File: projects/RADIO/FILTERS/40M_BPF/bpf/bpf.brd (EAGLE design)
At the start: 90 x 30 mm, 15 parts

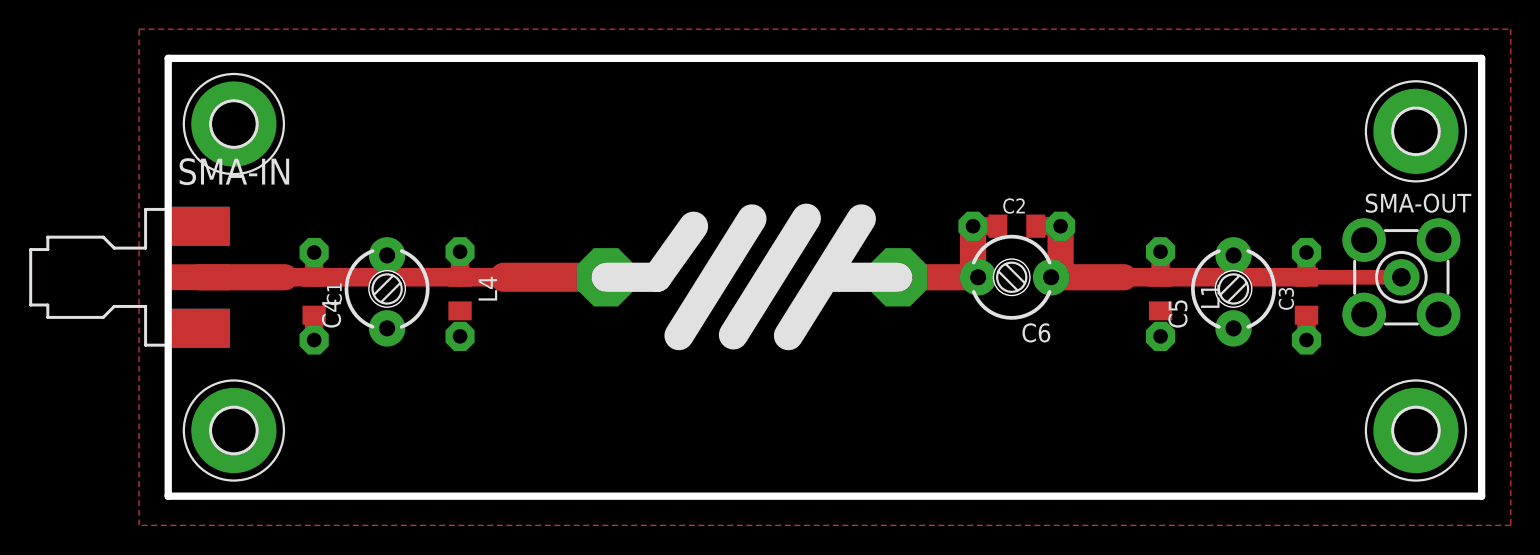
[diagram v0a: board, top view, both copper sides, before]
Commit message: update
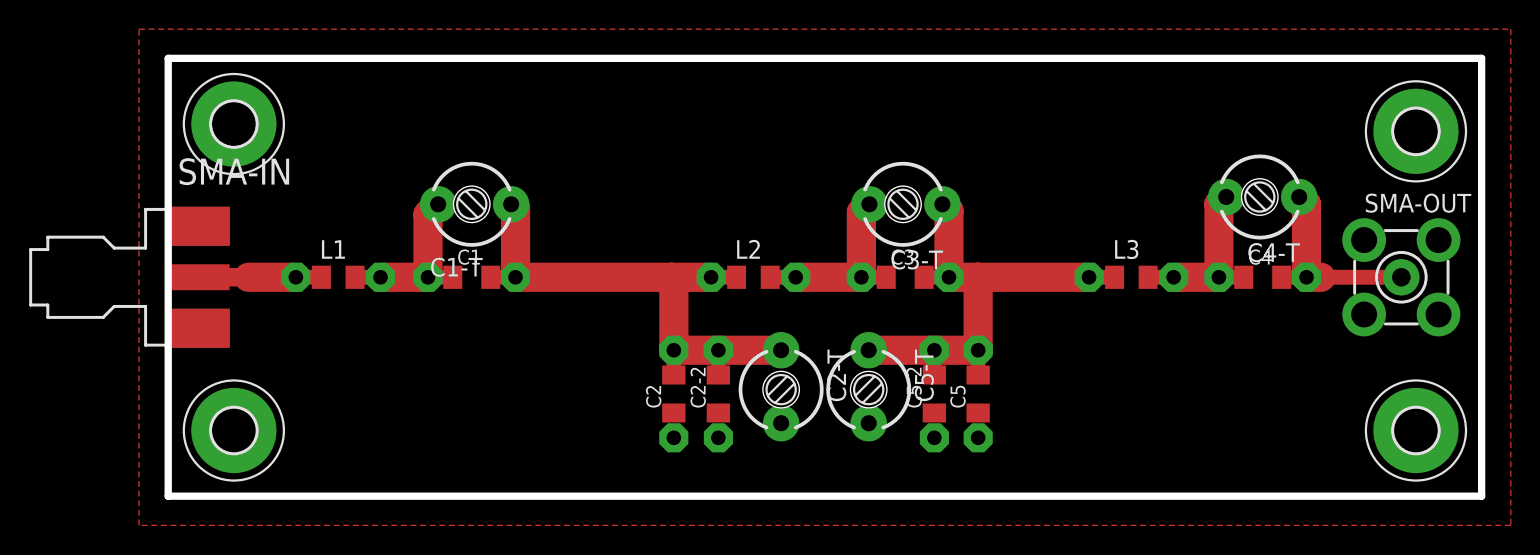
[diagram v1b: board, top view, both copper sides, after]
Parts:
- removed C6: (no value), mylib:CTRIM3050.505
- removed L4: (no value), mylib:M0805
- removed L5: (no value), mylib:L_WIRE16MM
- added C1-T, C2-T, C3-T, C4-T, C5-T: (no value), mylib:CTRIM3050.505
- added C2-2, C5-2: (no value), mylib:C0805K
- added L2, L3: (no value), mylib:M0805
- C4, C5: device mylib:CTRIM3050.505 -> mylib:C0805K
- moved C4 60.0 mm to (75.0, 15.0), turned to 0 degrees
- moved L1 56.4 mm to (11.7, 15.0), turned to 0 degrees
- moved C3 27.5 mm to (50.5, 15.0), turned to 0 degrees
- moved C2 26.2 mm to (34.6, 7.00), turned to 90 degrees
- moved C5 18.8 mm to (55.5, 7.00)
- moved C1 10.9 mm to (20.8, 15.0), turned to 0 degrees
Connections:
- removed net DIV: C2.1, C2.P$1, C6.2, L5.P$2
- removed net IN: C1.1, C1.P$1, C4.2, L4.1, L4.P$1, L5.P$1, SMA-IN.1
- removed net OUT: C2.2, C2.P$2, C3.2, C3.P$2, C5.2, C6.1, L1.1, L1.P$1, SMA-OUT.1
- new net N$1: L1.1, L1.P$1, SMA-IN.1
- new net N$2: C1-T.2, C1.1, C1.P$1, L1.2, L1.P$2
- new net N$3: C1-T.1, C1.2, C1.P$2, C2-2.2, C2-2.P$2, C2-T.1, C2.2, C2.P$2, L2.1, L2.P$1
- new net N$4: C3-T.2, C3.1, C3.P$1, L2.2, L2.P$2
- new net N$5: C3-T.1, C3.2, C3.P$2, C5-2.2, C5-2.P$2, C5-T.1, C5.2, C5.P$2, L3.1, L3.P$1
- new net N$6: C4-T.2, C4.1, C4.P$1, L3.2, L3.P$2
- new net N$7: C4-T.1, C4.2, C4.P$2, SMA-OUT.1
- net GND: now also C2-2.1, C2-2.P$1, C2-T.2, C2.1, C2.P$1, C5-2.1, C5-2.P$1, C5-T.2, C5.P$1; no longer C1.2, C1.P$2, C3.1, C3.P$1, C4.1, L1.2, L1.P$2, L4.2, L4.P$2
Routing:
- net N$3: track 0.00 -> 37.8 mm
- net OUT: track 34.3 -> 0.00 mm
- net N$5: track 0.00 -> 34.1 mm
- net IN: track 32.8 -> 0.00 mm
- net N$7: track 0.00 -> 13.9 mm
- net N$4: track 0.00 -> 13.2 mm
- net N$6: track 0.00 -> 12.3 mm
- net N$2: track 0.00 -> 12.0 mm
- net DIV: track 10.2 -> 0.00 mm
- net N$1: track 0.00 -> 8.38 mm
- net GND: track 3.40 -> 0.00 mm
